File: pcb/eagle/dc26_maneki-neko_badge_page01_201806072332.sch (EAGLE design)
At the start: 53 parts, among them T1 RK7002BMT116, U1 STM32F030C8T, U2 PAM2301CAAB330, U3 NPTC042KFMS-RC, U5 MIC2005A-1YM5-TR, U6 MIC2005A-1YM5-TR, X1 22-23-2021

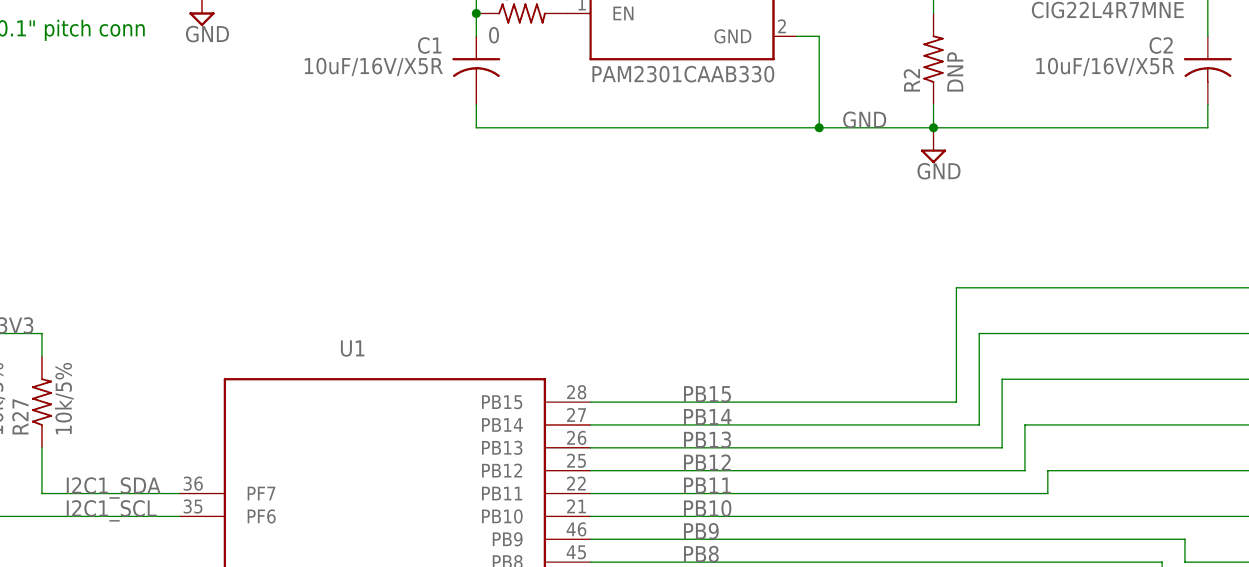
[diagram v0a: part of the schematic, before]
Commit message: completely regretting my decision to use eagle
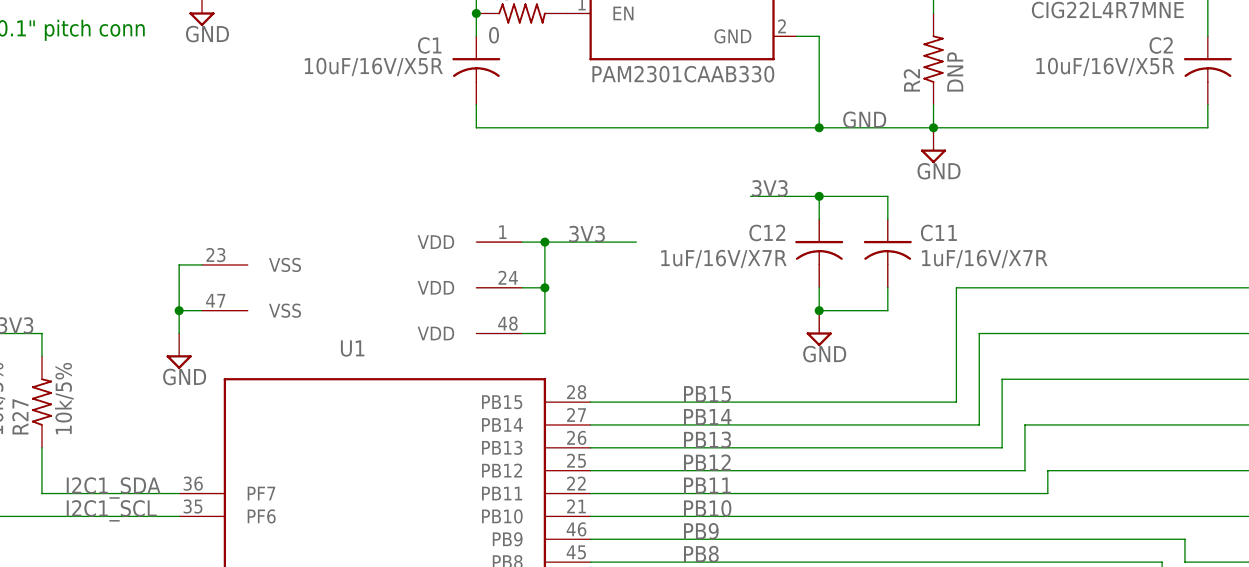
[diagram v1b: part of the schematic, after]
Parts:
- added C11, C12: 1uF/16V/X7R, rcl:C-USC0805
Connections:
- net 3V3: now also C11.1, C12.1, U1PWR.VDD@1, U1PWR.VDD@2, U1PWR.VDD@3
- net GND: now also C11.2, C12.2, U1PWR.VSS@1, U1PWR.VSS@2
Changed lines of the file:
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@@
 <part name="H3" library="dc26-shitty-addon" deviceset="SHITTY-ADDON-HEADER-MASTER" device=""/>
 <part name="U3" library="NPTC042KFMS-RC" deviceset="NPTC042KFMS-RC" device=""/>
+<part name="C11" library="rcl" library_urn="urn:adsk.eagle:library:334" deviceset="C-US" device="C0805" package3d_urn="urn:adsk.eagle:package:23617/2" value="1uF/16V/X7R"/>
+<part name="C12" library="rcl" library_urn="urn:adsk.eagle:library:334" deviceset="C-US" device="C0805" package3d_urn="urn:adsk.eagle:package:23617/2" value="1uF/16V/X7R"/>
+<part name="SUPPLY19" library="supply2" library_urn="urn:adsk.eagle:library:372" deviceset="GND" device=""/>
+<part name="SUPPLY20" library="supply2" library_urn="urn:adsk.eagle:library:372" deviceset="GND" device=""/>
 </parts>
 <sheets>
@@
 </plain>
 <instances>
-<instance part="U1" gate="MCU" x="-144.78" y="137.16"/>
+<instance part="U1" gate="MCU" x="-144.78" y="137.16" smashed="yes">
+<attribute name="NAME" x="-149.86" y="182.88" size="1.778" layer="95"/>
+<attribute name="VALUE" x="-149.86" y="91.44" size="1.778" layer="96"/>
+</instance>
 <instance part="X1" gate="-1" x="-172.72" y="226.06" rot="MR0"/>
 <instance part="X1" gate="-2" x="-172.72" y="223.52" rot="MR0"/>
@@
 <instance part="H3" gate="G$1" x="-223.52" y="149.86"/>
 <instance part="U3" gate="G$1" x="-10.16" y="68.58"/>
+<instance part="U1" gate="PWR" x="-147.32" y="190.5" rot="R270"/>
+<instance part="C11" gate="G$1" x="-88.9" y="195.58" smashed="yes" rot="MR0">
+<attribute name="NAME" x="-85.344" y="197.485" size="1.778" layer="95" rot="MR180"/>
+<attribute name="VALUE" x="-85.344" y="194.691" size="1.778" layer="96" rot="MR180"/>
+</instance>
+<instance part="C12" gate="G$1" x="-96.52" y="195.58" smashed="yes">
+<attribute name="NAME" x="-100.076" y="197.485" size="1.778" layer="95" rot="R180"/>
+<attribute name="VALUE" x="-100.076" y="194.691" size="1.778" layer="96" rot="R180"/>
+</instance>
+<instance part="SUPPLY19" gate="GND" x="-167.64" y="182.88"/>
+<instance part="SUPPLY20" gate="GND" x="-96.52" y="185.42"/>
 </instances>
 <busses>
@@
 <label x="-241.3" y="149.86" size="1.778" layer="95"/>
 </segment>
+<segment>
+<pinref part="SUPPLY19" gate="GND" pin="GND"/>
+<pinref part="U1" gate="PWR" pin="VSS@1"/>
+<wire x1="-167.64" y1="185.42" x2="-167.64" y2="187.96" width="0.1524" layer="91"/>
+<wire x1="-167.64" y1="187.96" x2="-167.64" y2="193.04" width="0.1524" layer="91"/>
+<wire x1="-167.64" y1="193.04" x2="-165.1" y2="193.04" width="0.1524" layer="91"/>
+<pinref part="U1" gate="PWR" pin="VSS@2"/>
+<wire x1="-165.1" y1="187.96" x2="-167.64" y2="187.96" width="0.1524" layer="91"/>
+<junction x="-167.64" y="187.96"/>
+</segment>
+<segment>
+<pinref part="C12" gate="G$1" pin="2"/>
+<pinref part="SUPPLY20" gate="GND" pin="GND"/>
+<wire x1="-96.52" y1="190.5" x2="-96.52" y2="187.96" width="0.1524" layer="91"/>
+<pinref part="C11" gate="G$1" pin="2"/>
+<wire x1="-88.9" y1="190.5" x2="-88.9" y2="187.96" width="0.1524" layer="91"/>
+<wire x1="-88.9" y1="187.96" x2="-96.52" y2="187.96" width="0.1524" layer="91"/>
+<junction x="-96.52" y="187.96"/>
+</segment>
 </net>
 <net name="VBAT" class="0">
@@
 <label x="-241.3" y="152.4" size="1.778" layer="95"/>
 </segment>
+<segment>
+<pinref part="U1" gate="PWR" pin="VDD@3"/>
+<wire x1="-129.54" y1="185.42" x2="-127" y2="185.42" width="0.1524" layer="91"/>
+<wire x1="-127" y1="185.42" x2="-127" y2="190.5" width="0.1524" layer="91"/>
+<pinref part="U1" gate="PWR" pin="VDD@1"/>
+<wire x1="-127" y1="190.5" x2="-127" y2="195.58" width="0.1524" layer="91"/>
+<wire x1="-127" y1="195.58" x2="-129.54" y2="195.58" width="0.1524" layer="91"/>
+<pinref part="U1" gate="PWR" pin="VDD@2"/>
+<wire x1="-129.54" y1="190.5" x2="-127" y2="190.5" width="0.1524" layer="91"/>
+<junction x="-127" y="190.5"/>
+<wire x1="-127" y1="195.58" x2="-116.84" y2="195.58" width="0.1524" layer="91"/>
+<label x="-124.46" y="195.58" size="1.778" layer="95"/>
+<junction x="-127" y="195.58"/>
+</segment>
+<segment>
+<pinref part="C12" gate="G$1" pin="1"/>
+<wire x1="-96.52" y1="198.12" x2="-96.52" y2="200.66" width="0.1524" layer="91"/>
+<wire x1="-96.52" y1="200.66" x2="-104.14" y2="200.66" width="0.1524" layer="91"/>
+<pinref part="C11" gate="G$1" pin="1"/>
+<wire x1="-88.9" y1="198.12" x2="-88.9" y2="200.66" width="0.1524" layer="91"/>
+<wire x1="-88.9" y1="200.66" x2="-96.52" y2="200.66" width="0.1524" layer="91"/>
+<junction x="-96.52" y="200.66"/>
+<label x="-104.14" y="200.66" size="1.778" layer="95"/>
+</segment>
 </net>
